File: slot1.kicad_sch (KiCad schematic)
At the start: 1 part

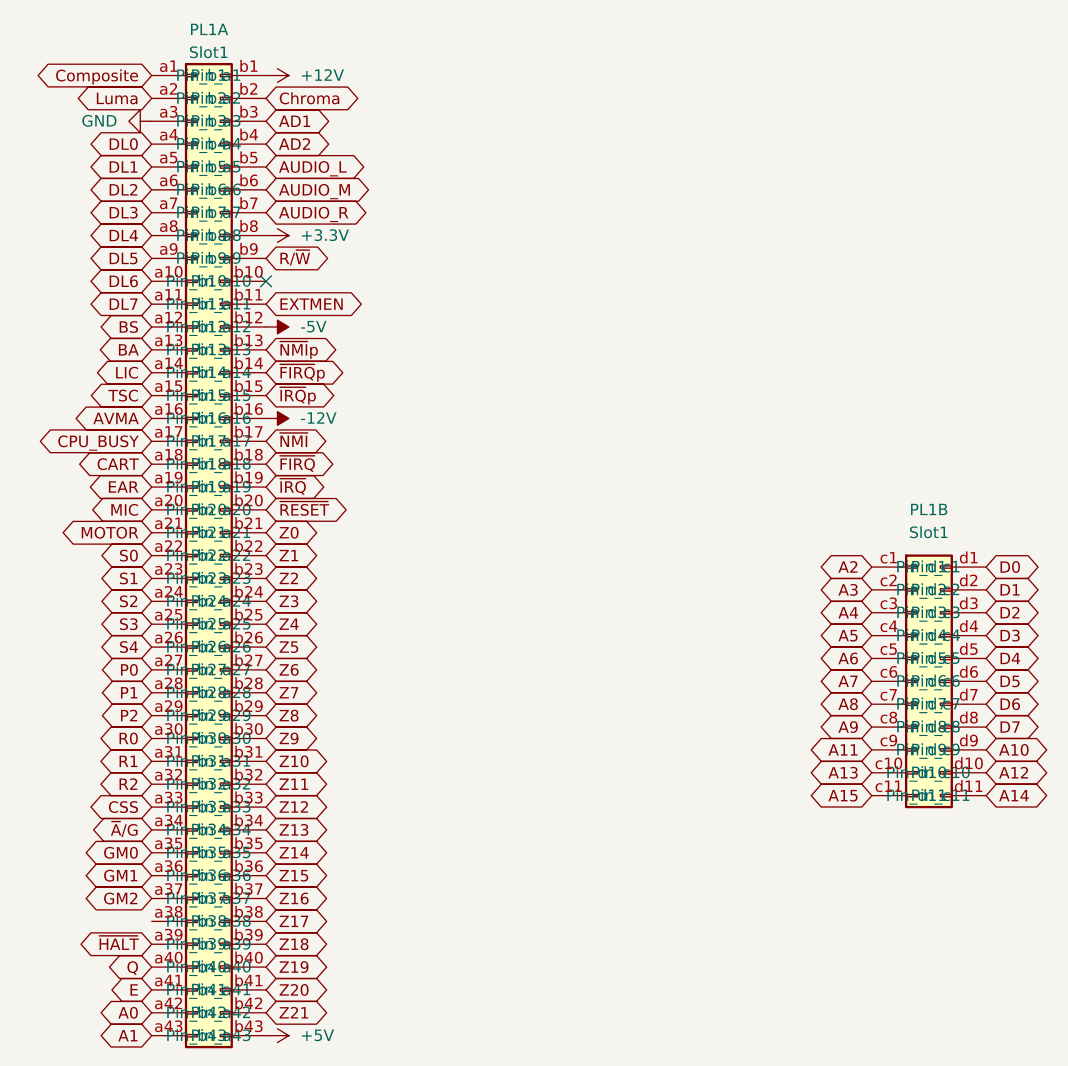
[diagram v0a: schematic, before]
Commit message: board layout
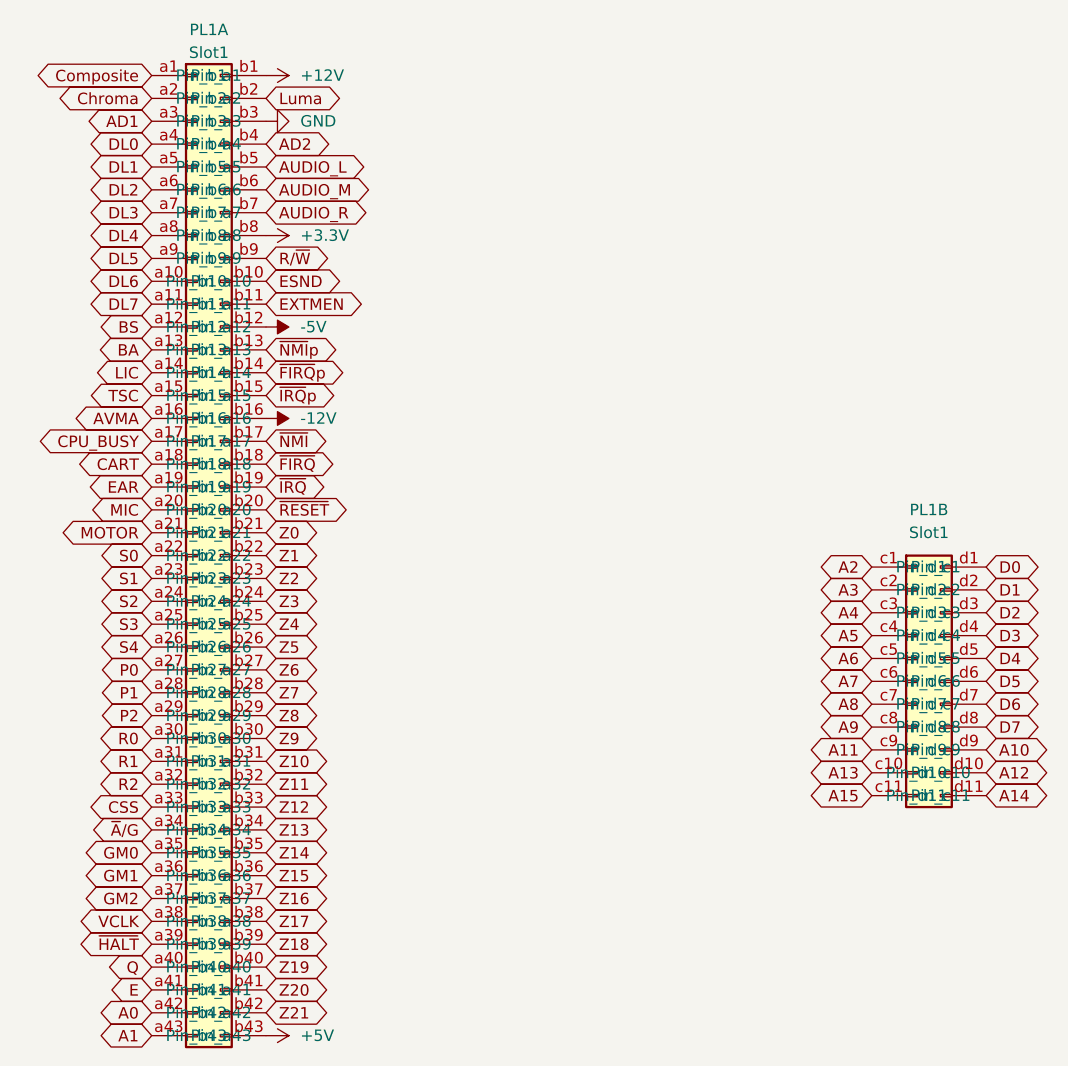
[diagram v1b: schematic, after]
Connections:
- net AD1: now also PL1.a3 (Pin_a3); no longer PL1.b3 (Pin_b3)
- net Chroma: now also PL1.a2 (Pin_a2); no longer PL1.b2 (Pin_b2)
- net GND: now also PL1.b3 (Pin_b3); no longer PL1.a3 (Pin_a3)
- net Luma: now also PL1.b2 (Pin_b2); no longer PL1.a2 (Pin_a2)
- net VCLK: now reaches PL1.a38 (Pin_a38)
- net ESND: now reaches PL1.b10 (Pin_b10)
- no-connect marks 1 -> 0
